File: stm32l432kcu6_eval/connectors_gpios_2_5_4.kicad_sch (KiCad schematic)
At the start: 17 parts, among them J1 Conn_01x04_Pin, J2 Conn_01x20_Pin, J4 Conn_01x20_Pin

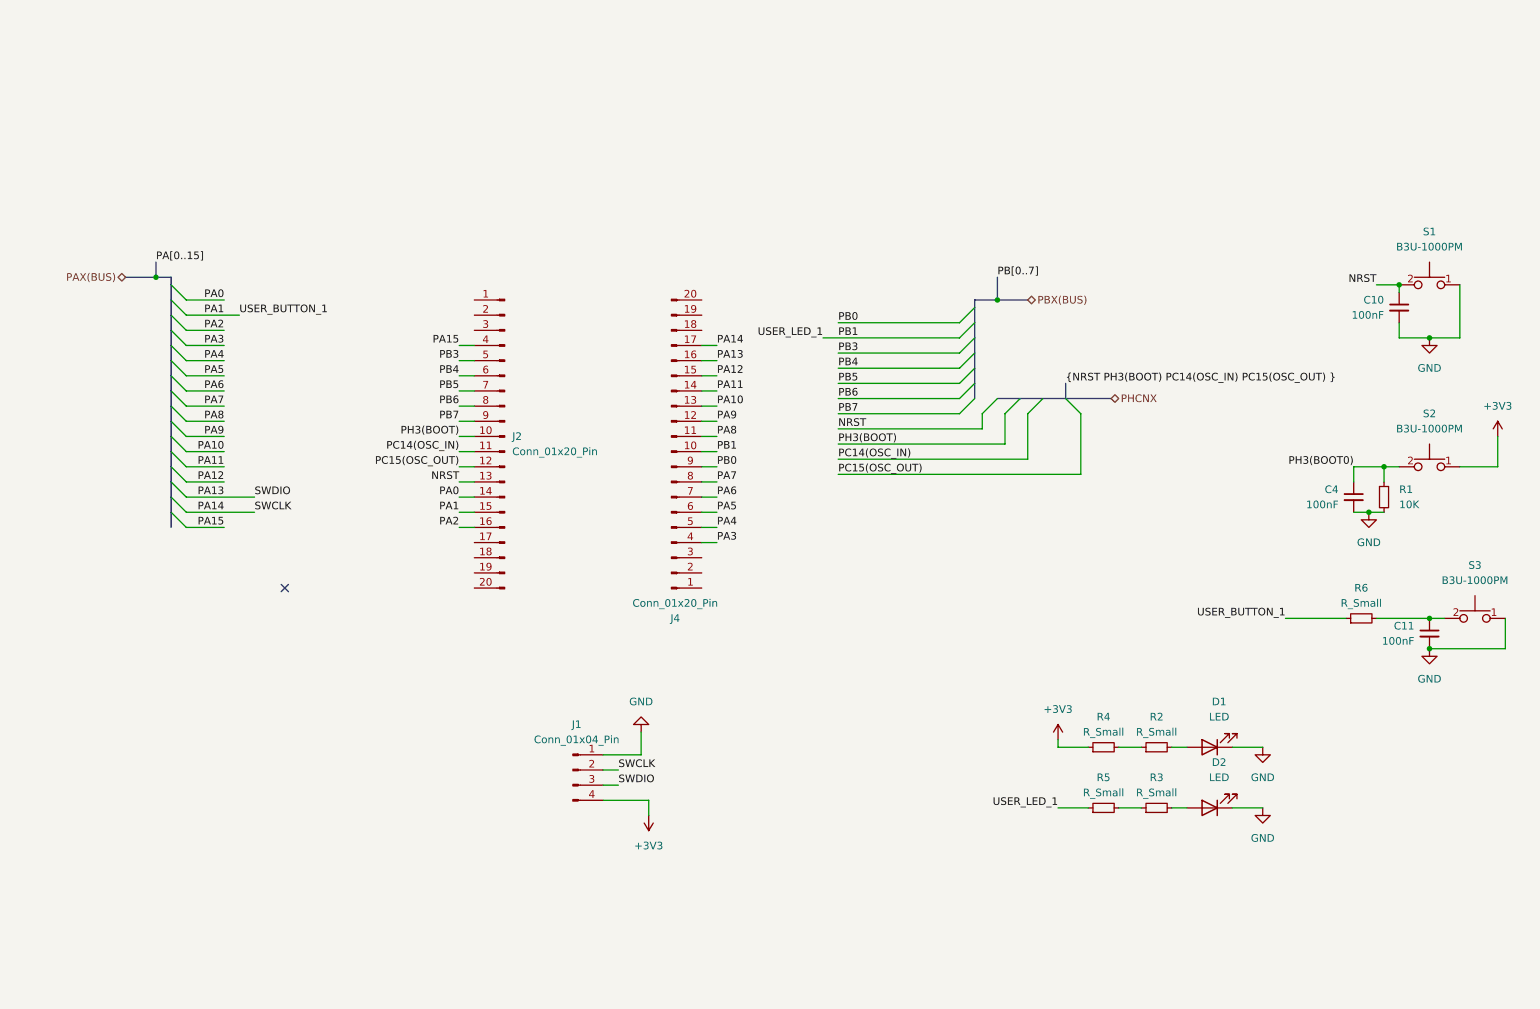
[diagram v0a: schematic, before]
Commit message: organisation save 2
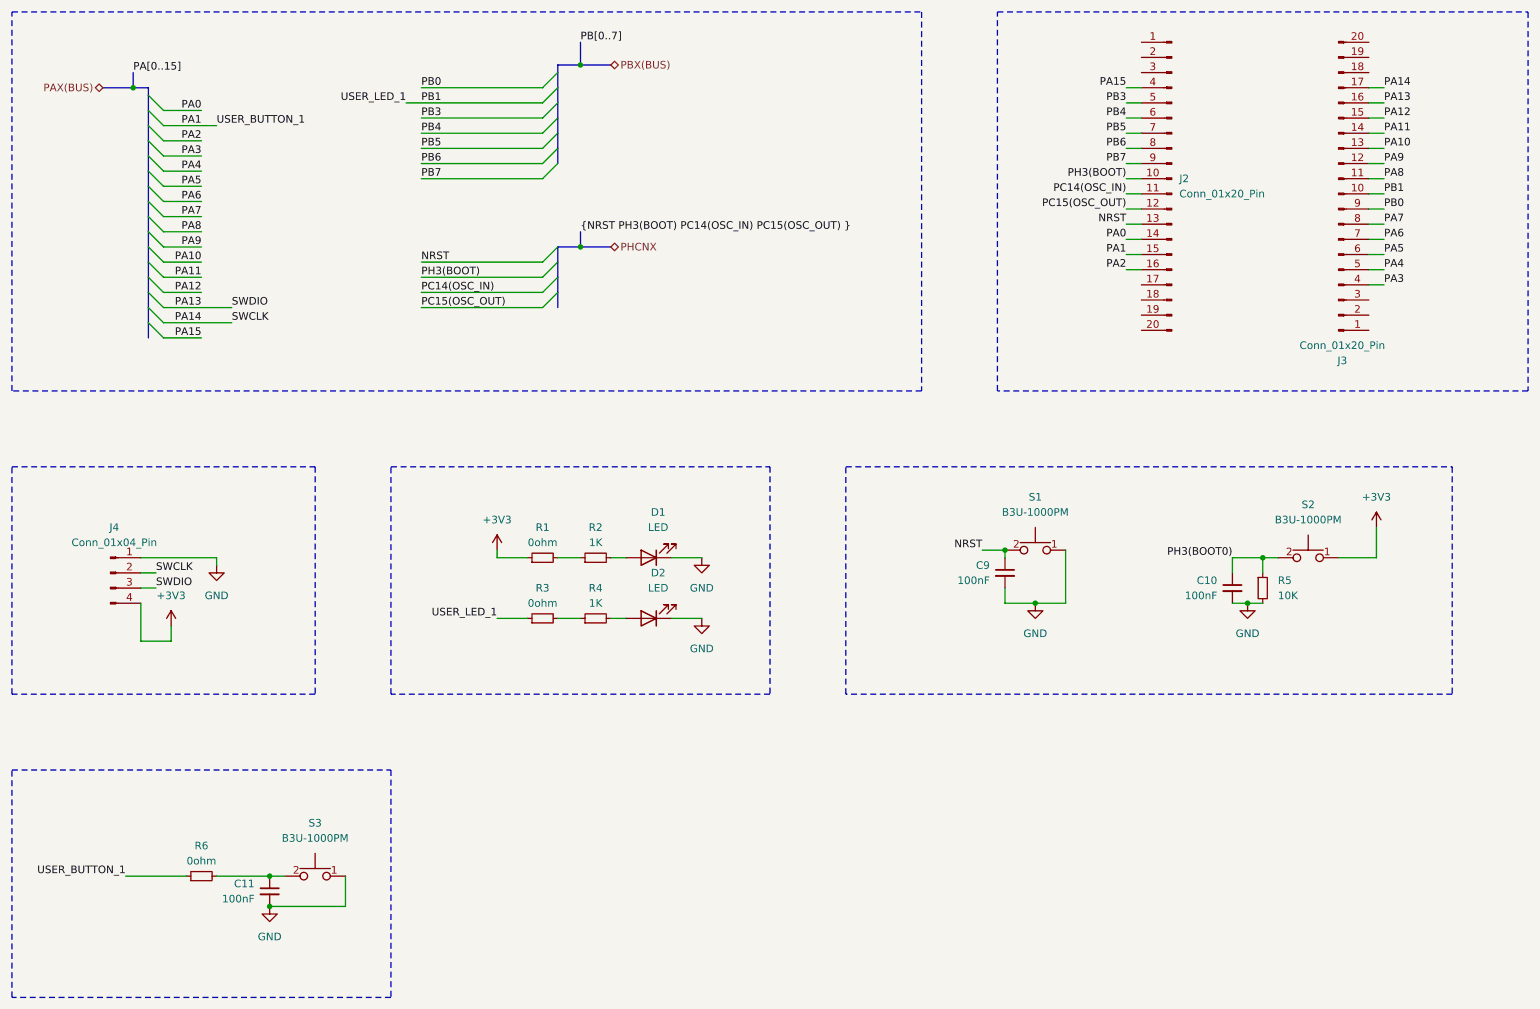
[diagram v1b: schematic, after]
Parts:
- R1: renamed from R4; value R_Small -> 0ohm
- R2: value R_Small -> 1K
- R3: renamed from R5; value R_Small -> 0ohm
- R4: renamed from R3; value R_Small -> 1K
- R6: value R_Small -> 0ohm
- renumbered C4 to C10, C10 to C9, J4 to J3, J1 to J4, R1 to R5
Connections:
- no-connect marks 1 -> 0
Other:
- moved on the sheet: C10, C11, C9, D1, D2, J2, J3, J4, R1, R2, R3, R4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
